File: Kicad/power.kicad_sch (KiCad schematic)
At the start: 31 parts, among them J7 22112042

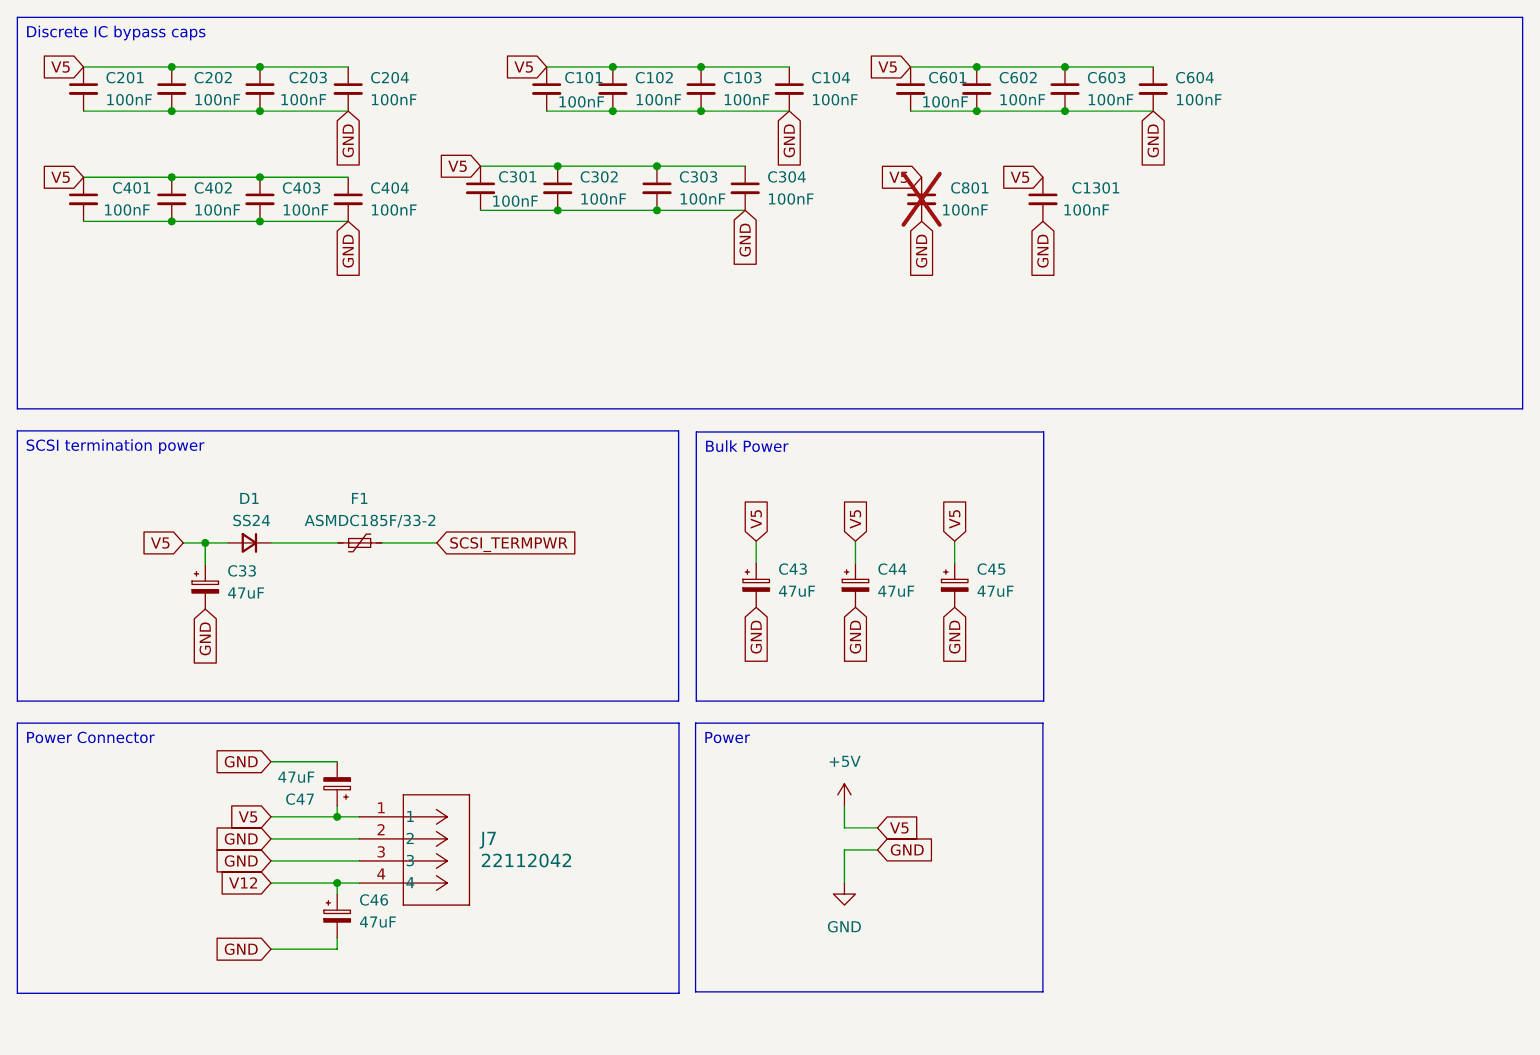
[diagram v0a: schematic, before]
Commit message: Clean up schematics
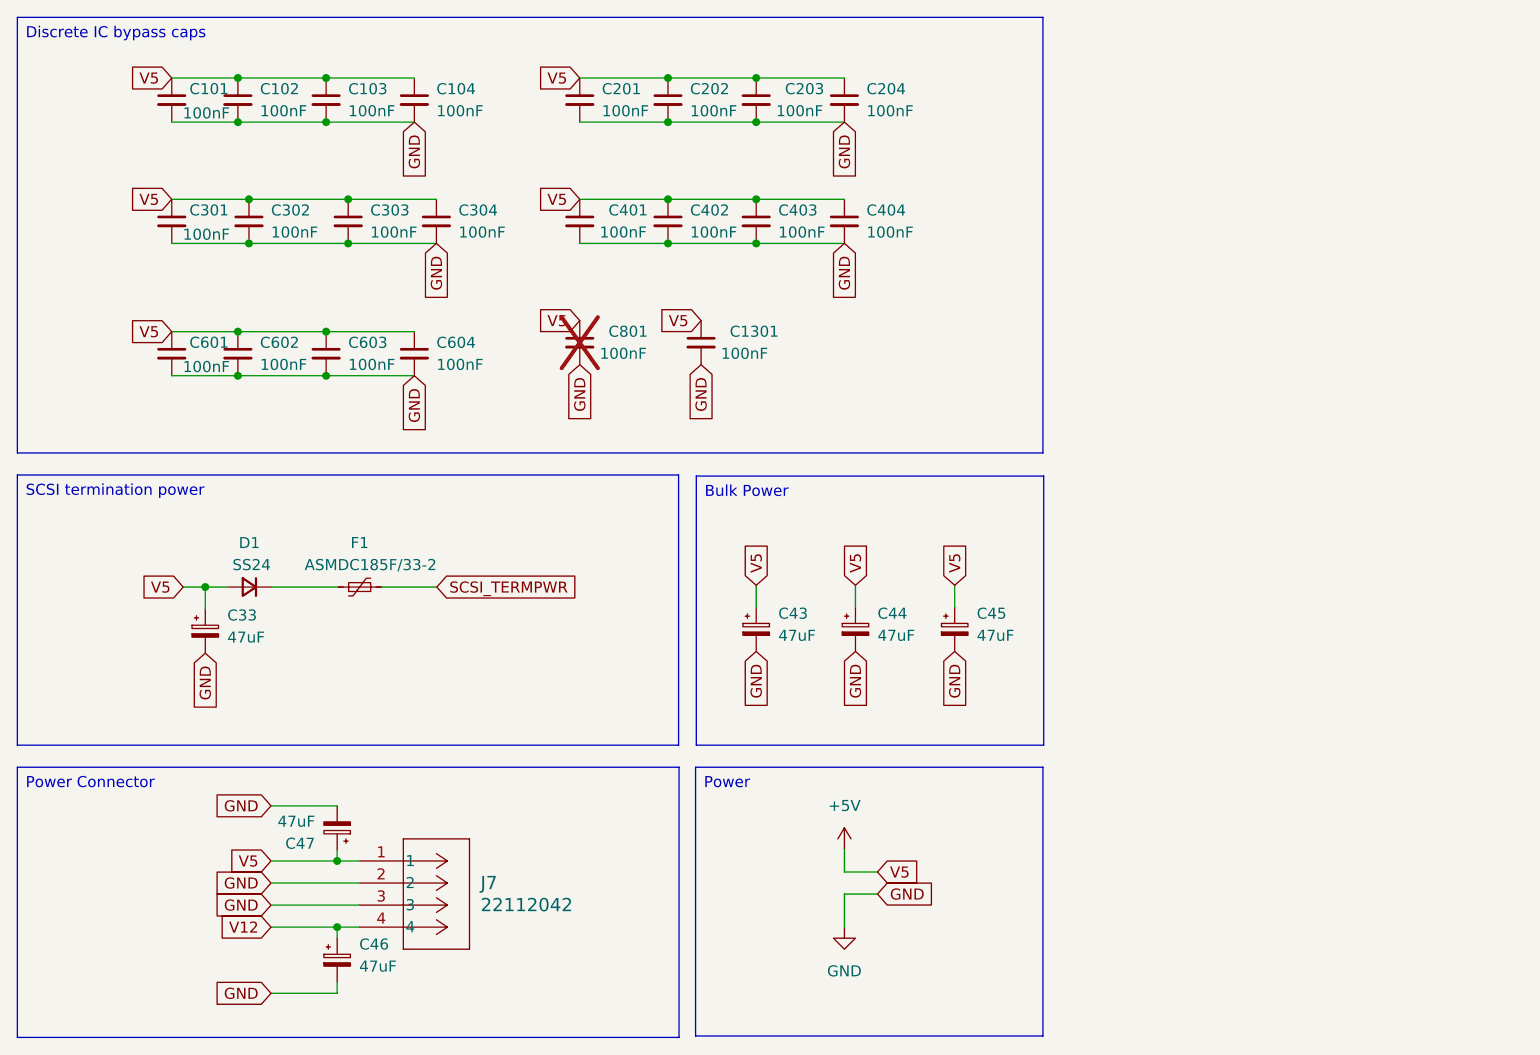
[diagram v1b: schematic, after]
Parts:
- F1: LCSC Part # C3761950 -> C135379
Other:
- moved on the sheet: C101, C102, C103, C104, C1301, C201, C202, C203, C204, C301, C302, C303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
